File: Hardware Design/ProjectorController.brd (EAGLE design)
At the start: 55.5 x 38.1 mm, 13 parts, among them J1 5747844-4, J2 Cap Buttons, J3 Prog, J4 Prog/Run, J5 10118194-0001LF, U1 ESP-WROOM-32, U2 SP3232EEN-L

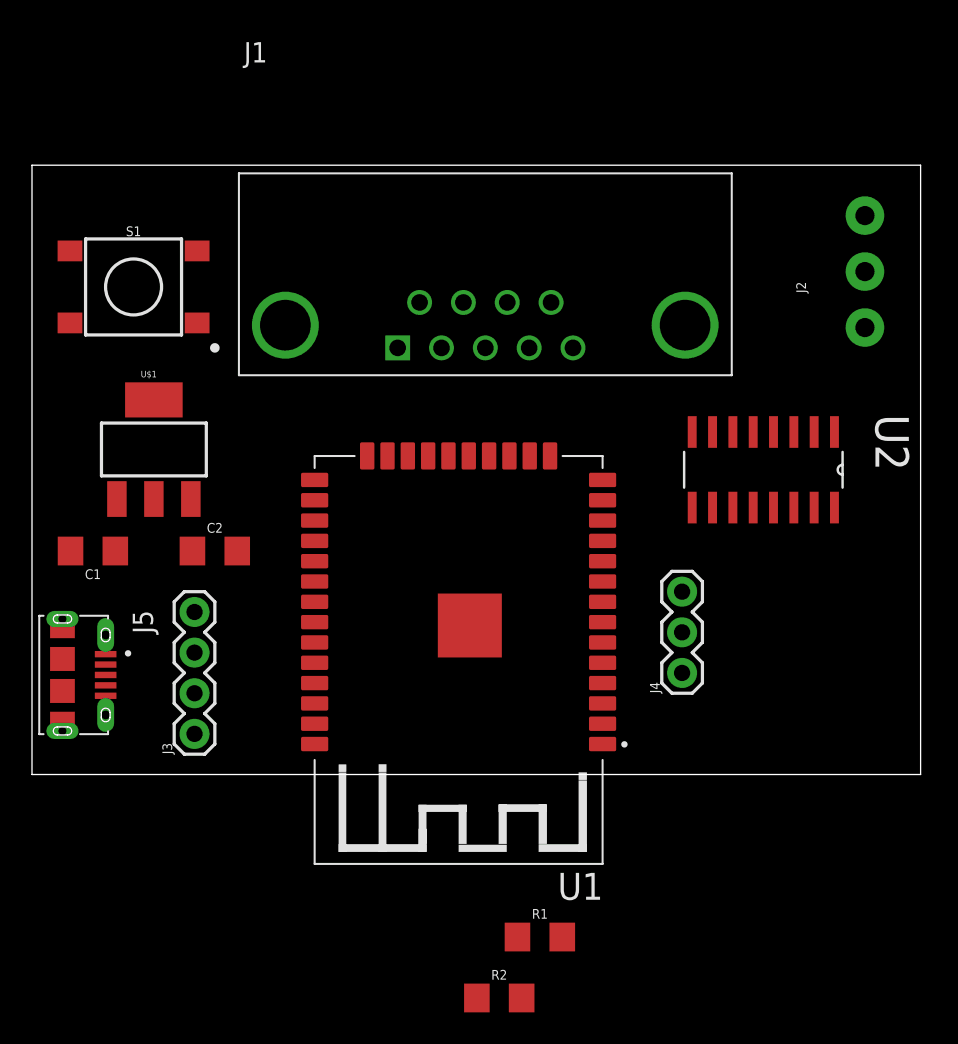
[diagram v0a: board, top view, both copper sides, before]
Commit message: Progress on board layout PC-13
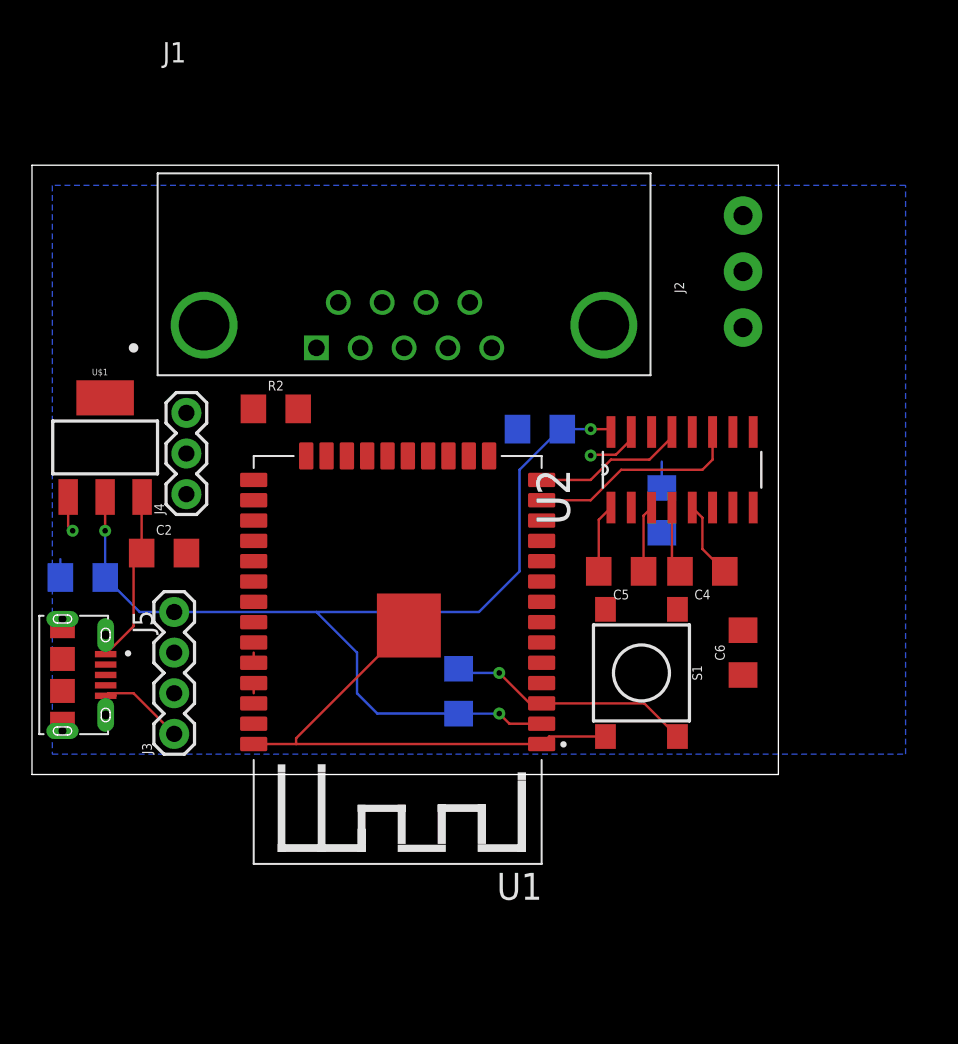
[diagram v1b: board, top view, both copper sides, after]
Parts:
- added C3, C4, C5, C6, C7: 0.1uF, SparkFun-Capacitors:1206
- moved S1 39.9 mm to (41.9, 49.5), turned to 270 degrees
- moved R2 39.4 mm to (19.1, 66.0)
- moved J4 32.9 mm to (13.5, 60.7)
- moved R1 16.2 mm to (30.5, 48.4), flipped to the bottom, turned to 90 degrees
- moved J2 7.62 mm to (48.3, 71.1)
- moved J1 5.08 mm to (21.6, 69.8)
- moved U2 5.08 mm to (44.5, 62.2), turned to 90 degrees
- moved U1 3.81 mm to (26.7, 53.3)
- moved C2 3.18 mm to (12.1, 57.0)
- moved U$1 3.05 mm to (8.38, 63.6)
- moved C1 1.77 mm to (6.99, 55.5), flipped to the bottom, turned to 0 degrees
- moved J3 1.27 mm to (12.7, 45.7)
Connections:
- removed net V+: U2.2
- removed net V-: U2.6
- new net N$12: C5.2, U2.1
- new net N$14: C5.1, U2.3
- new net N$15: C4.2, U2.4
- new net N$16: C4.1, U2.5
- new net N$17: C7.2, U2.2
- new net N$19: C6.2, U2.6
- net 3V3: now also C3.2
- net GND: now also C3.1, C6.1, C7.1
- net N$7: now also J3.2; no longer J3.3
- net N$8: now also J3.3; no longer J3.2
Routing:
- net 3V3: track 0.00 -> 65.3 mm, vias 0 -> 3
- net GND: track 0.00 -> 48.8 mm, vias 0 -> 2
- net N$4: track 0.00 -> 15.4 mm, vias 0 -> 1
- net N$9: track 0.00 -> 13.5 mm
- net 5V: track 0.00 -> 11.1 mm
- net N$13: track 0.00 -> 9.58 mm
- net N$16: track 0.00 -> 4.83 mm
- net N$12: track 0.00 -> 4.30 mm
- net N$15: track 0.00 -> 4.20 mm
- net N$14: track 0.00 -> 4.20 mm
- net N$7: track 0.00 -> 0.64 mm
- net N$8: track 0.00 -> 0.63 mm
- added copper zone on layer 16, net GND
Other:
- board size 55.5 x 38.1 mm -> 46.7 x 38.1 mm
